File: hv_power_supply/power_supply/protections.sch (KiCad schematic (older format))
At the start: 12 parts, among them K1 DBR71210(NC), K2 LI12-1A85(NO), Q2 SSM3K333R, SW1 SW_Push_SPST_NO

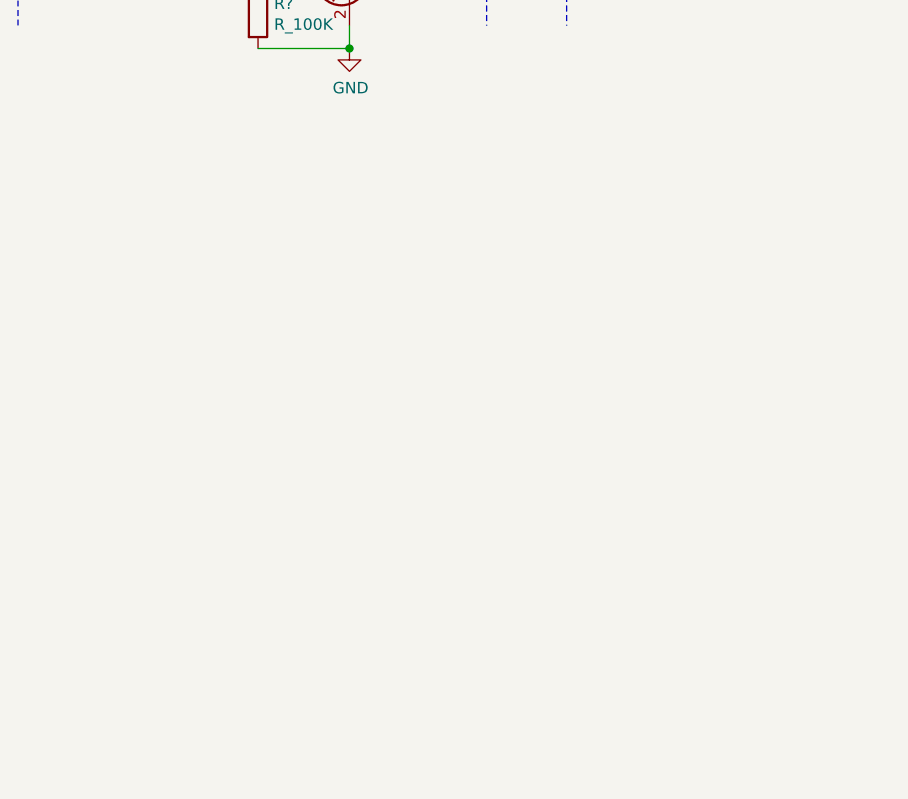
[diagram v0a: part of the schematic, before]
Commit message: minor changes
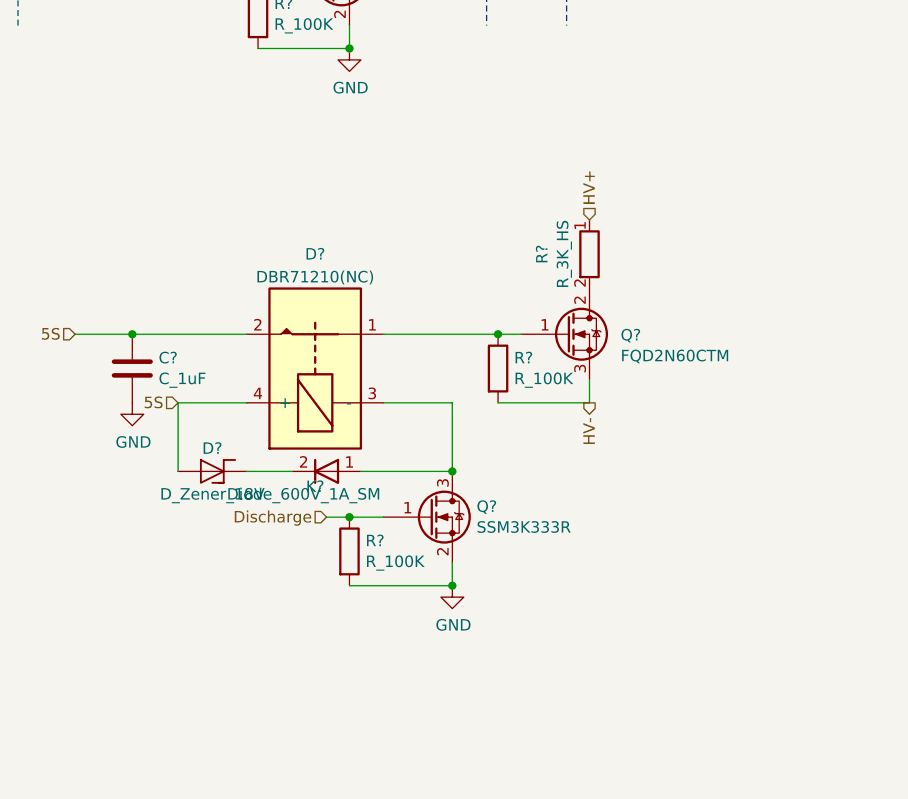
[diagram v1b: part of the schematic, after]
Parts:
- added C?: C_1uF, footprints:C_0805_OEM, symbol formula:C_1uF
- added D?: D_Zener_18V, footprints:DO-214AA, symbol formula:D_Zener_18V
- added D?: Diode_600V_1A_SM, footprints:Diode_600V_1A_SM, symbol formula:Diode_600V_1A_SM
- added K?: DBR71210(NC), footprints:D-Series_Cynergy_Relay, symbol formula:DBR71210(NC)
- added Q?: FQD2N60CTM, footprints:DPAK229P990X239-4N, symbol formula:FQD2N60CTM
- added Q?: SSM3K333R, footprints:SOT-23F, symbol formula:SSM3K333R
- added R?: R_3K_HS, footprints:R_3k_HS_TO247, symbol formula:R_3K_HS
- added R? (x2): R_100K, footprints:R_0805_OEM, symbol formula:R_100K
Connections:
- net Discharge: now also Q?.1 (G), R?.1
- net GND: now also C?.2, Q?.2 (S), R?.2
- net HV+: now also R?.1
- net HV-: now also Q?.3, R?.2
- new net: K?.1, Q?.1, R?.1
- new net: D?.1, K?.3 (-), Q?.3 (D)
- new net: Q?.2, R?.2
- new net: D?.1 (K), D?.2
- new net 5S: C?.1, D?.2 (A), K?.2, K?.4 (+)
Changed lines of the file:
@@
 	1650 2200 1550 2200
 Connection ~ 1650 2200
+Wire Wire Line
+	850  3750 1100 3750
+$Comp
+L formula:C_1uF C?
+U 1 1 5FD57537
+P 1100 3950
+F 0 "C?" H 1215 4046 50  0000 L CNN
+F 1 "C_1uF" H 1215 3955 50  0000 L CNN
+F 2 "footprints:C_0805_OEM" H 1138 4550 50  0001 C CNN
+F 3 "https://www.yageo.com/upload/media/product/productsearch/datasheet/mlcc/UPY-GPHC_Y5V_6.3V-to-50V_9.pdf" H 1125 4800 50  0001 C CNN
+F 4 "https://www.digikey.com/product-detail/en/yageo/CC0805ZKY5V9BB105/311-1909-1-ND/5195811#images" H 1525 4450 60  0001 C CNN "PurchasingLink"
+	1    1100 3950
+	1    0    0    -1
+$EndComp
+Text HLabel 850  3750 0    50   Input ~ 0
+5S
+Connection ~ 2500 4850
+Wire Wire Line
+	2500 4750 2500 4850
+Wire Wire Line
+	2050 4850 2500 4850
+Text HLabel 1950 4550 0    50   Input ~ 0
+Discharge
+Wire Wire Line
+	2050 4550 1950 4550
+Connection ~ 2050 4550
+Wire Wire Line
+	2200 4550 2050 4550
+$Comp
+L formula:R_100K R?
+U 1 1 5FD49978
+P 2050 4700
+F 0 "R?" H 2120 4746 50  0000 L CNN
+F 1 "R_100K" H 2120 4655 50  0000 L CNN
+F 2 "footprints:R_0805_OEM" H 1980 4700 50  0001 C CNN
+F 3 "https://industrial.panasonic.com/cdbs/www-data/pdf/RDA0000/AOA0000C304.pdf" H 2130 4700 50  0001 C CNN
+F 4 "DK" H 2050 4700 60  0001 C CNN "MFN"
+F 5 "P100KCCT-ND" H 2050 4700 60  0001 C CNN "MPN"
+F 6 "https://www.digikey.com/product-detail/en/panasonic-electronic-components/ERJ-6ENF1003V/P100KCCT-ND/119551" H 2530 5100 60  0001 C CNN "PurchasingLink"
+	1    2050 4700
+	1    0    0    -1
+$EndComp
+$Comp
+L power:GND #PWR?
+U 1 1 5FD491A0
+P 2500 4850
+F 0 "#PWR?" H 2500 4600 50  0001 C CNN
+F 1 "GND" H 2505 4677 50  0000 C CNN
+F 2 "" H 2500 4850 50  0001 C CNN
+F 3 "" H 2500 4850 50  0001 C CNN
+	1    2500 4850
+	1    0    0    -1
+$EndComp
+$Comp
+L formula:SSM3K333R Q?
+U 1 1 5FD46161
+P 2400 4550
+F 0 "Q?" H 2606 4596 50  0000 L CNN
+F 1 "SSM3K333R" H 2606 4505 50  0000 L CNN
+F 2 "footprints:SOT-23F" H 2600 4475 50  0001 L CIN
+F 3 "https://drive.google.com/drive/folders/0B-V-iZf33Y4GNzhDQTJZanJRbVk" H 2600 4625 50  0001 L CNN
+F 4 "DK" H 2900 4925 60  0001 C CNN "MFN"
+F 5 "SSM3K333RLFCT-ND" H 2800 4825 60  0001 C CNN "MPN"
+F 6 "https://www.digikey.com/product-detail/en/toshiba-semiconductor-and-storage/SSM3K333RLF/SSM3K333RLFCT-ND/3522391" H 2700 4725 60  0001 C CNN "PurchasingLink"
+	1    2400 4550
+	1    0    0    -1
+$EndComp
+Text HLabel 1300 4050 0    50   Input ~ 0
+5S
+Text HLabel 3100 4050 3    50   Output ~ 0
+HV-
+Text HLabel 3100 3250 1    50   Input ~ 0
+HV+
+$Comp
+L formula:R_3K_HS R?
+U 1 1 5FD26F91
+P 3100 3400
+F 0 "R?" V 2893 3400 50  0000 C CNN
+F 1 "R_3K_HS" V 2984 3400 50  0000 C CNN
+F 2 "footprints:R_3k_HS_TO247" H 3030 3400 50  0001 C CNN
+F 3 "http://dpk3n3gg92jwt.cloudfront.net/domains/ohmite/pdf/acl_ap101.pdf" H 3180 3400 50  0001 C CNN
+F 4 "DK" H 3100 3400 60  0001 C CNN "MFN"
+F 5 "AP1013KJ-ND" H 3100 3400 60  0001 C CNN "MPN"
+F 6 "https://www.digikey.com/product-detail/en/ohmite/AP101-3K-J/AP101-3K-J-ND/5878525" H 3580 3800 60  0001 C CNN "PurchasingLink"
+F 7 "345-1223-ND" V 3680 3900 60  0001 C CNN "MPN2"
+F 8 "https://www.digikey.com/product-detail/en/wakefield-vette/657-15ABPEN/345-1223-ND/3945700" V 3780 4000 60  0001 C CNN "PurchasingLink2"
+	1    3100 3400
+	1    0    0    -1
+$EndComp
+$Comp
+L formula:FQD2N60CTM Q?
+U 1 1 5FD240E6
+P 3100 3800
+F 0 "Q?" H 3236 3846 50  0000 L CNN
+F 1 "FQD2N60CTM" H 3236 3755 50  0000 L CNN
+F 2 "footprints:DPAK229P990X239-4N" H 3090 4260 50  0001 C CNN
+F 3 "https://www.onsemi.com/pub/Collateral/FQU2N60C-D.PDF" H 3100 3800 50  0001 C CNN
+F 4 "ON Semiconductor" H 3100 3800 50  0001 C CNN "MFN"
+F 5 "FDB33N25TM" H 3100 3800 50  0001 C CNN "MPN"
+F 6 "https://www.digikey.com/en/products/detail/on-semiconductor/FQD2N60CTM/1053993" H 3100 3800 50  0001 C CNN "Purchasing Link"
+	1    3100 3800
+	1    0    0    -1
+$EndComp
+$Comp
+L formula:DBR71210(NC) K?
+U 1 1 5FCF383E
+P 1900 3850
+F 0 "K?" V 1333 3850 50  0000 C CNN
+F 1 "DBR71210(NC)" V 2250 3850 50  0000 C CNN
+F 2 "footprints:D-Series_Cynergy_Relay" H 2350 3800 50  0001 L CNN
+F 3 "https://www.cynergy3.com/sites/default/files/D%20series%202016_5.pdf" H 2350 3500 50  0001 L CNN
+F 4 "DK" H 2750 4400 60  0001 C CNN "MFN"
+F 5 "725-1049-ND" H 2650 4300 60  0001 C CNN "MPN"
+F 6 "https://www.digikey.com/product-detail/en/cynergy-3/DBR71210/725-1049-ND/752025" H 2850 4500 60  0001 C CNN "PurchasingLink"
+	1    1900 3850
+	0    -1   -1   0
+$EndComp
+Connection ~ 1100 3750
+Wire Wire Line
+	1100 3750 1600 3750
+$Comp
+L power:GND #PWR?
+U 1 1 5FD6CC93
+P 1100 4050
+F 0 "#PWR?" H 1100 3800 50  0001 C CNN
+F 1 "GND" H 1105 3877 50  0000 C CNN
+F 2 "" H 1100 4050 50  0001 C CNN
+F 3 "" H 1100 4050 50  0001 C CNN
+	1    1100 4050
+	1    0    0    -1
+$EndComp
+$Comp
+L formula:D_Zener_18V D?
+U 1 1 5FD6F617
+P 1450 4350
+F 0 "D?" H 1450 4250 50  0000 C CNN
+F 1 "D_Zener_18V" H 1450 4450 50  0000 C CNN
+F 2 "footprints:DO-214AA" H 1350 4350 50  0001 C CNN
+F 3 "http://www.mccsemi.com/up_pdf/SMBJ5338B-SMBJ5388B(SMB).pdf" H 1450 4450 50  0001 C CNN
+F 4 "DK" H 1650 4650 60  0001 C CNN "MFN"
+F 5 "SMBJ5355B-TPMSCT-ND" H 1550 4550 60  0001 C CNN "MPN"
+F 6 "https://www.digikey.com/products/en?keywords=SMBJ5355B-TPMSCT-ND" H 1850 4850 60  0001 C CNN "PurchasingLink"
+	1    1450 4350
+	-1   0    0    1
+$EndComp
+$Comp
+L formula:Diode_600V_1A_SM D?
+U 1 1 5FD6FE42
+P 1950 4350
+F 0 "D?" H 2000 3400 50  0000 C CNN
+F 1 "Diode_600V_1A_SM" H 2050 4450 50  0000 C CNN
+F 2 "footprints:Diode_600V_1A_SM" H 1900 4500 50  0001 C CNN
+F 3 "https://www.st.com/content/ccc/resource/technical/document/datasheet/c7/d5/fe/c4/56/21/41/02/CD00005135.pdf/files/CD00005135.pdf/jcr:content/translations/en.CD00005135.pdf" H 1900 4500 50  0001 C CNN
+F 4 "https://www.digikey.com/product-detail/en/stmicroelectronics/STTH1R06A/497-3765-1-ND/691935" H 1950 4550 50  0001 C CNN "Purchasing Link"
+	1    1950 4350
+	-1   0    0    1
+$EndComp
+Wire Wire Line
+	2200 4050 2500 4050
+Wire Wire Line
+	2500 4050 2500 4350
+Wire Wire Line
+	2500 4350 2100 4350
+Connection ~ 2500 4350
+Wire Wire Line
+	1800 4350 1600 4350
+Wire Wire Line
+	1300 4350 1300 4050
+Wire Wire Line
+	1300 4050 1600 4050
+$Comp
+L formula:R_100K R?
+U 1 1 5FEA809A
+P 2700 3900
+F 0 "R?" H 2770 3946 50  0000 L CNN
+F 1 "R_100K" H 2770 3855 50  0000 L CNN
+F 2 "footprints:R_0805_OEM" H 2630 3900 50  0001 C CNN
+F 3 "https://industrial.panasonic.com/cdbs/www-data/pdf/RDA0000/AOA0000C304.pdf" H 2780 3900 50  0001 C CNN
+F 4 "DK" H 2700 3900 60  0001 C CNN "MFN"
+F 5 "P100KCCT-ND" H 2700 3900 60  0001 C CNN "MPN"
+F 6 "https://www.digikey.com/product-detail/en/panasonic-electronic-components/ERJ-6ENF1003V/P100KCCT-ND/119551" H 3180 4300 60  0001 C CNN "PurchasingLink"
+	1    2700 3900
+	1    0    0    -1
+$EndComp
+Wire Wire Line
+	2200 3750 2700 3750
+Connection ~ 2700 3750
+Wire Wire Line
+	2700 3750 2800 3750
+Wire Wire Line
+	2700 4050 3100 4050
+Wire Wire Line
+	3100 3950 3100 4050
 $EndSCHEMATC

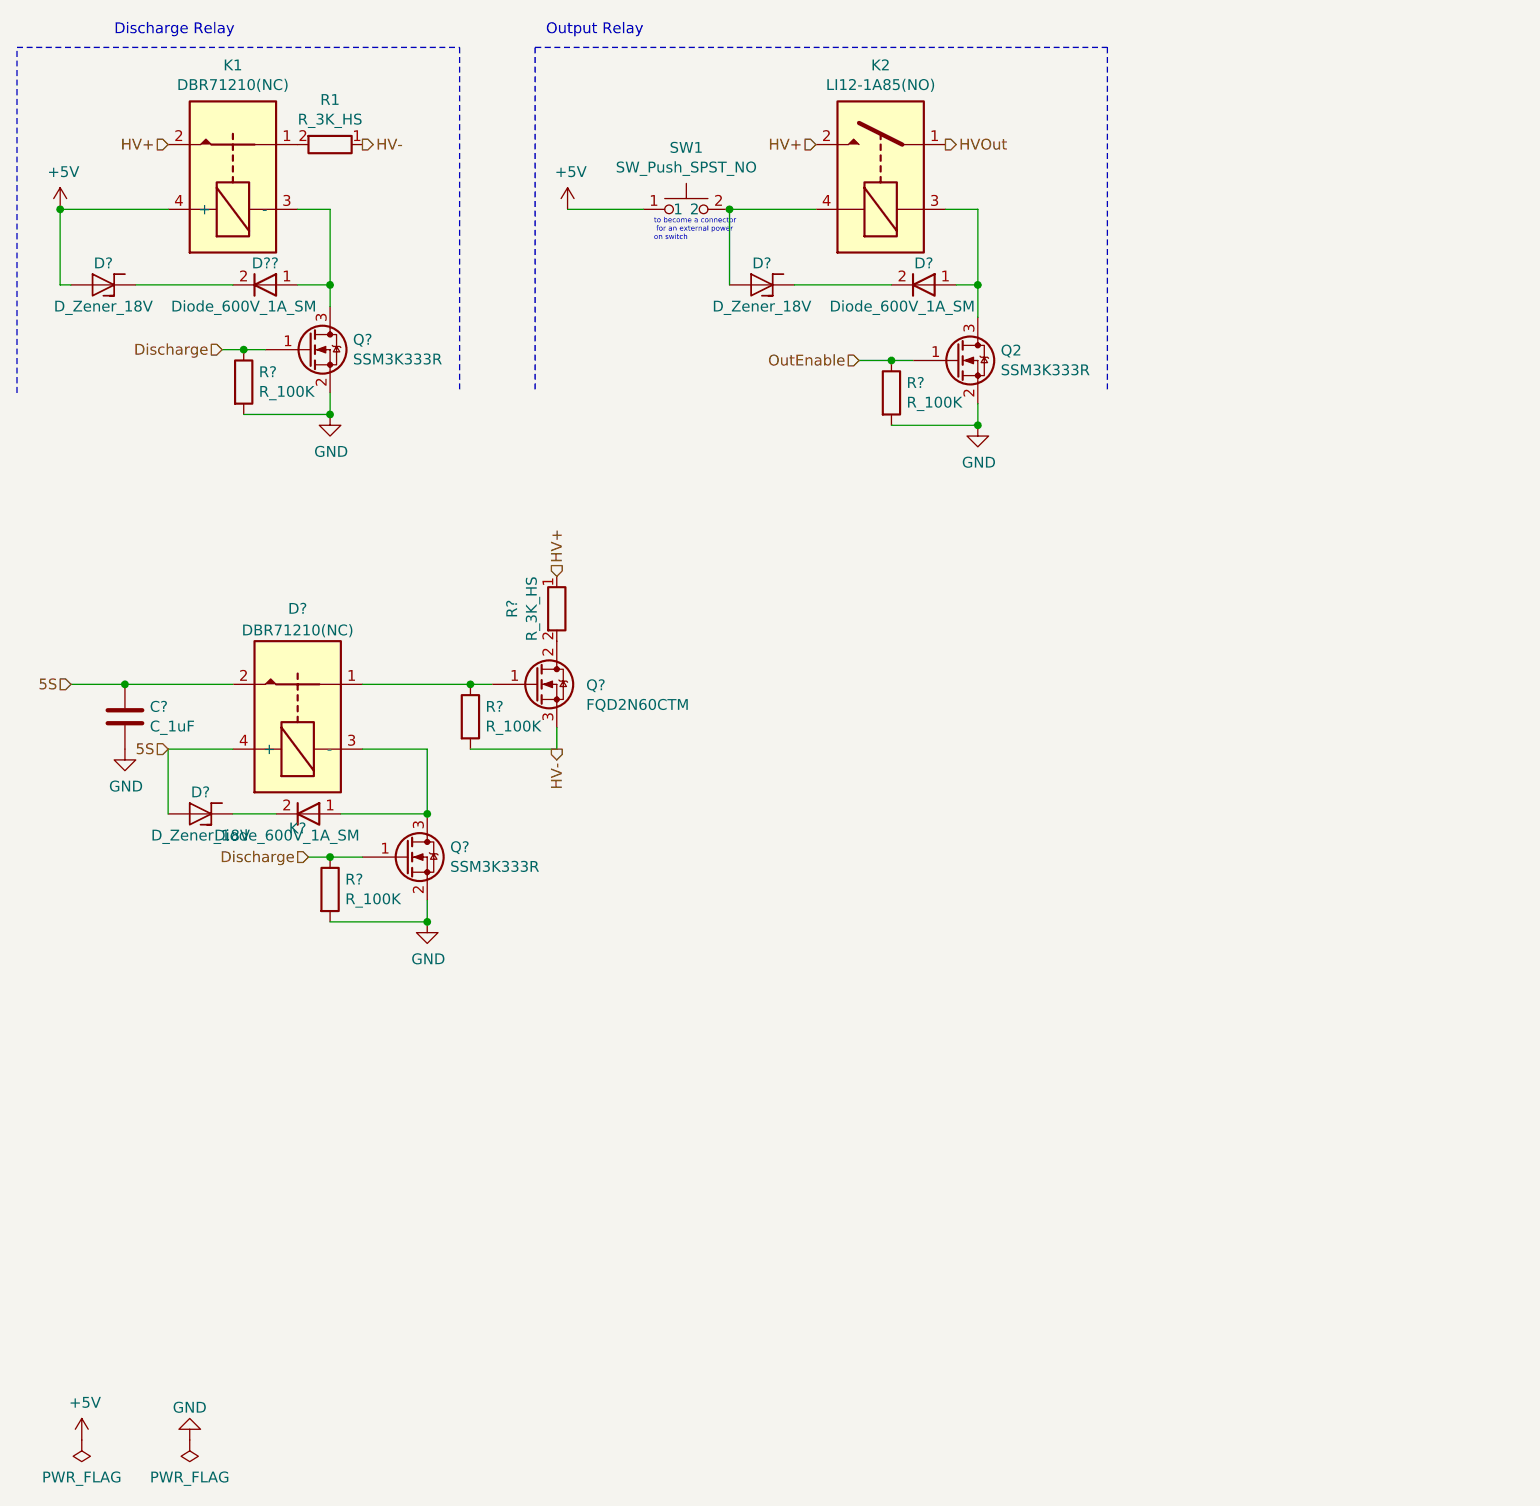
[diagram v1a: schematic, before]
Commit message: minor changes
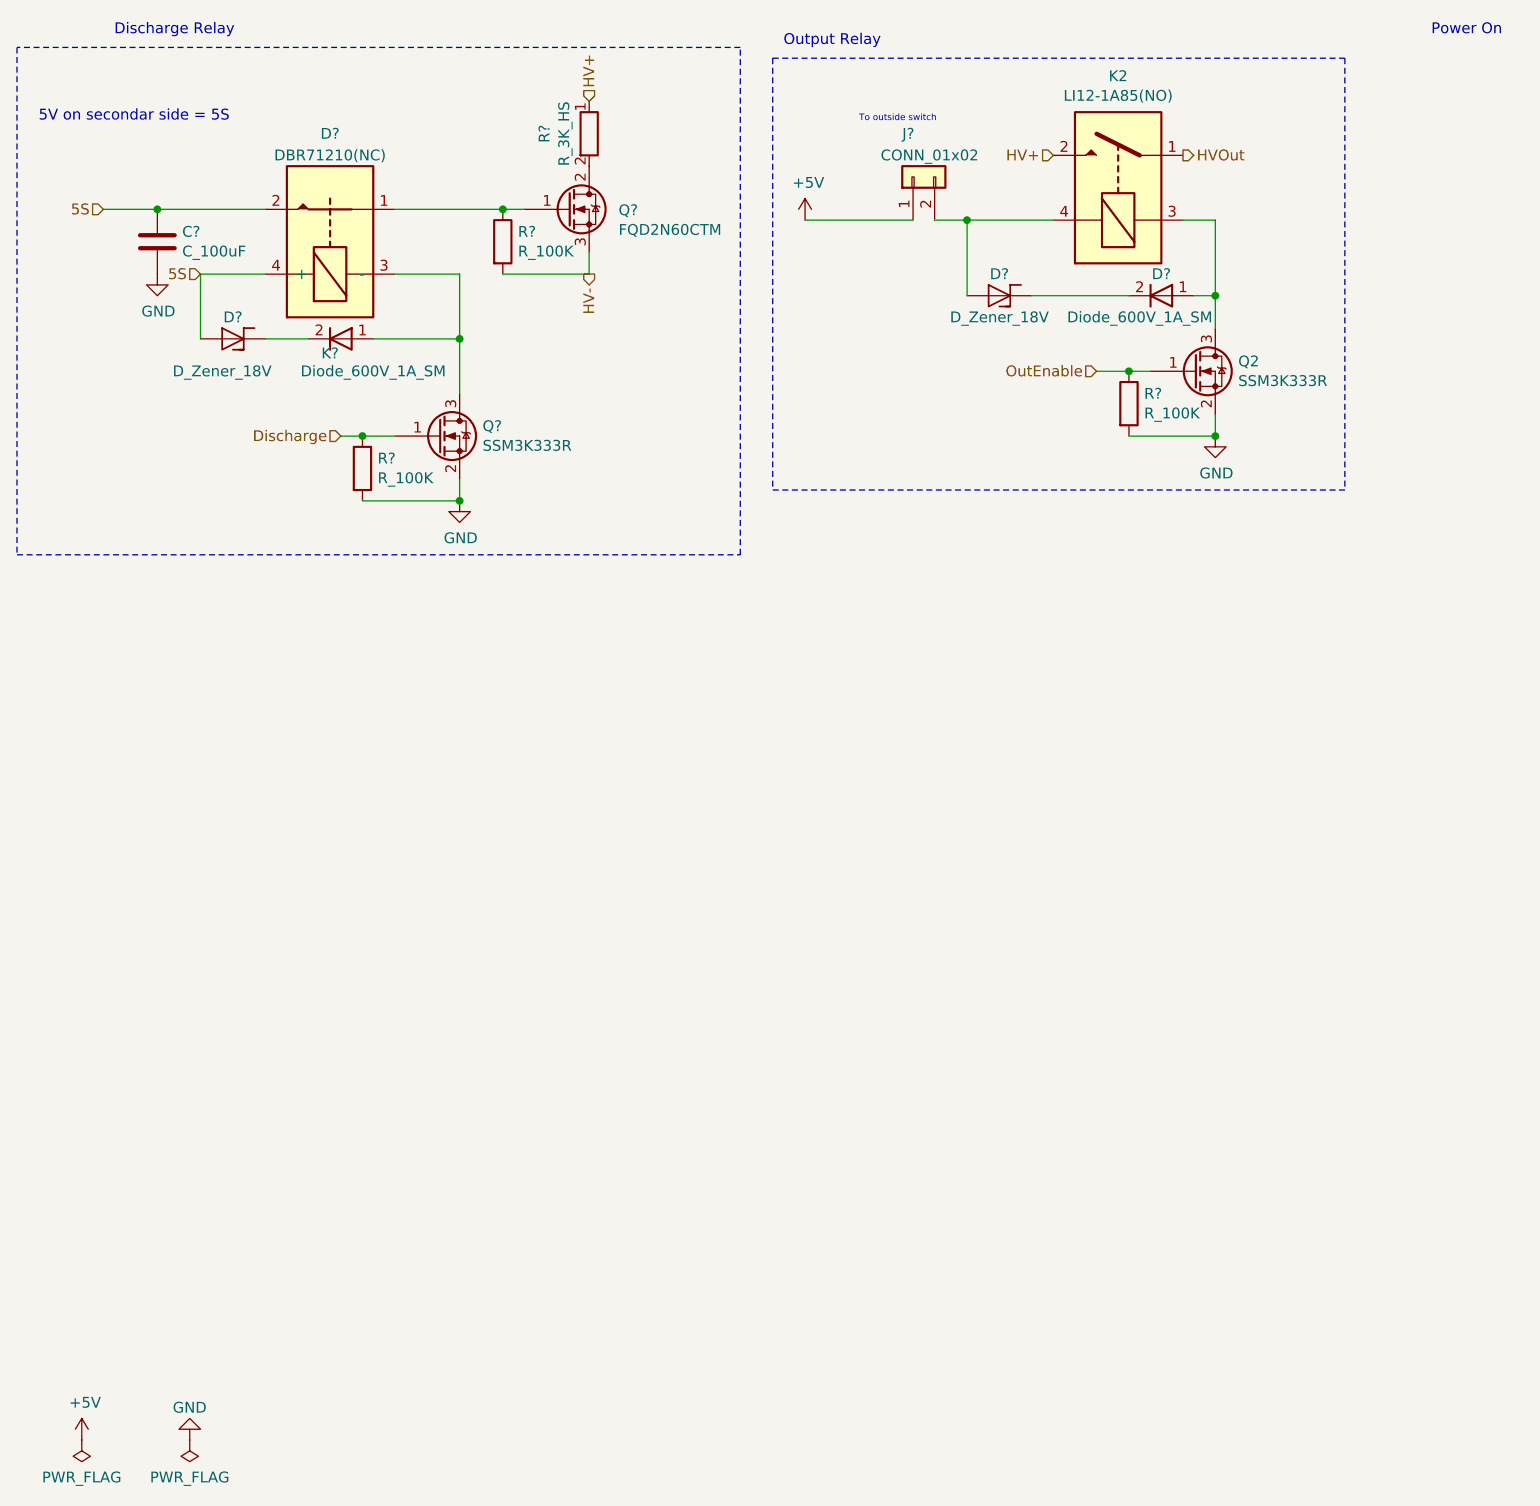
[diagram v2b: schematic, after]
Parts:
- removed C?: C_1uF, footprints:C_0805_OEM, symbol formula:C_1uF
- removed D?: D_Zener_18V, footprints:DO-214AA, symbol formula:D_Zener_18V
- removed D??: Diode_600V_1A_SM, footprints:Diode_600V_1A_SM, symbol formula:Diode_600V_1A_SM
- removed K1: DBR71210(NC), footprints:D-Series_Cynergy_Relay, symbol formula:DBR71210(NC)
- removed Q?: SSM3K333R, footprints:SOT-23F, symbol formula:SSM3K333R
- removed R1: R_3K_HS, footprints:R_3k_HS_TO247, symbol formula:R_3K_HS
- removed R? (x2): R_100K, footprints:R_0805_OEM, symbol formula:R_100K
- removed SW1: SW_Push_SPST_NO, footprints:SW_B3U-1000P_4.2x1.7mm, symbol formula:SW_Push_SPST_NO
- added C?: C_100uF, footprints:C_1812_4532Metric, symbol formula:C_100uF
- added J?: CONN_01x02, Connector_PinHeader_2.54mm:PinHeader_1x02_P2.54mm_Vertical, symbol formula:CONN_01x02
- added R?: R_100K, footprints:R_0805_OEM, symbol formula:R_100K
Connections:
- net +5V: now also J?.1 (Pin_1)
- net 5S: now also C?.1
- net GND: now also C?.2
- net HV-: now also R?.2
- net at D?.2 (A), K2.4: now also J?.2 (Pin_2)
- net at K?.1, Q?.1: now also R?.1
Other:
- note added: "5V on secondar side = 5S"
- note added: "Power On"
- note added: "To outside switch"
- note removed: "to become a connector\n for an external power \non switch"
- moved on the sheet: D?, K2, K?, Q2, Q?, R?
